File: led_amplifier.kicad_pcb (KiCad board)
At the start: 2 copper layers, 59 x 58.1 mm, 10 parts, among them J1 Conn_01x08_Female, J2 Conn_01x08_Female, Q1 IRF3205, Q2 IRF3205, Q3 IRF3205, Q4 IRF3205

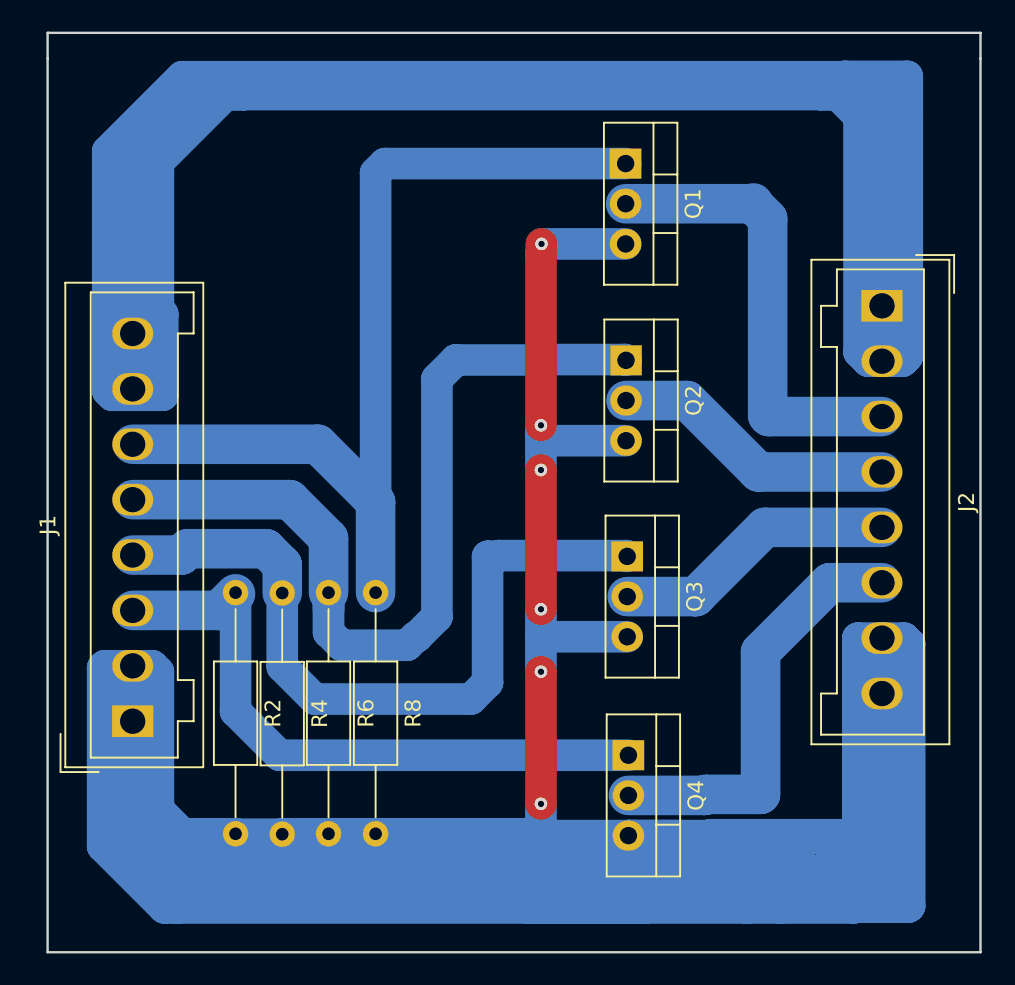
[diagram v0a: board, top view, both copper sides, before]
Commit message: Update...
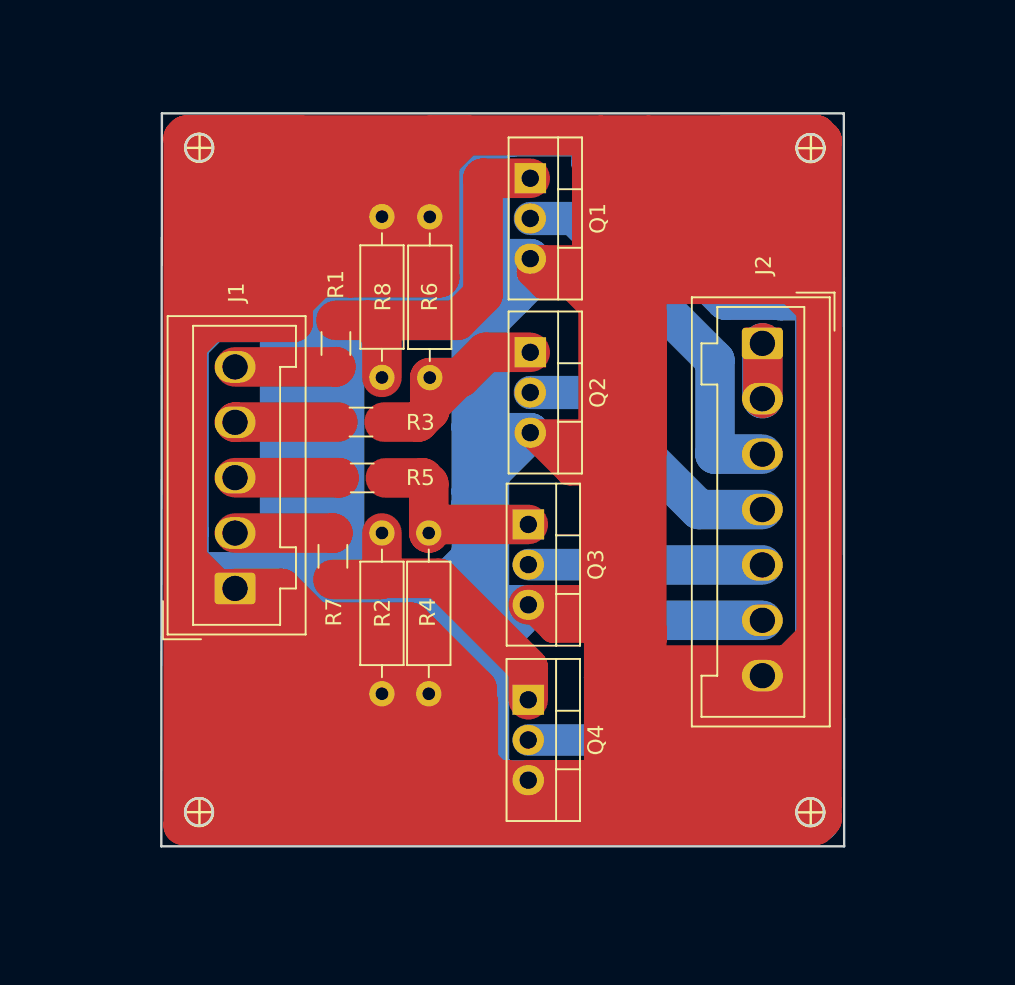
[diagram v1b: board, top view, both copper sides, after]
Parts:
- added R1: R, Resistor_SMD:R_1206_3216Metric, F.Cu at (151.9, 69.4)
- added R3: R, Resistor_SMD:R_1206_3216Metric, F.Cu at (153.5, 74.3)
- added R5: R, Resistor_SMD:R_1206_3216Metric, F.Cu at (153.6, 77.9)
- added R7: R, Resistor_SMD:R_1206_3216Metric, F.Cu at (151.8, 82.8)
- J1: value Conn_01x08_Female -> Conn_01x05; footprint Connector_Wago:Wago_734-138_1x08_P3.50mm_Vertical -> Connector_Wago:Wago_734-135_1x05_P3.50mm_Vertical
- J2: value Conn_01x08_Female -> Conn_01x07_Female; footprint Connector_Wago:Wago_734-138_1x08_P3.50mm_Vertical -> Connector_Wago:Wago_734-137_1x07_P3.50mm_Vertical
- R2, R4, R6, R8: footprint Resistor_THT:R_Axial_DIN0207_L6.3mm_D2.5mm_P15.24mm_Horizontal -> Resistor_THT:R_Axial_DIN0207_L6.3mm_D2.5mm_P10.16mm_Horizontal
- moved R6 15.0 mm to (157.9, 71.5), turned to 90 degrees
- moved R8 13.6 mm to (154.9, 71.5), turned to 90 degrees
- moved J1 10.6 mm to (145.6, 84.9)
- moved R4 10.0 mm to (157.8, 81.4)
- moved R2 9.99 mm to (154.9, 81.4)
- moved J2 7.92 mm to (178.9, 69.4)
- moved Q4 7.23 mm to (164.1, 91.9)
- moved Q3 6.57 mm to (164.1, 80.8)
- moved Q1 6.10 mm to (164.2, 58.9)
- moved Q2 6.07 mm to (164.2, 69.9)
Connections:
- J1 pad 2: Net-(J1-Pad1) -> Net-(J1-Pad2)
- J2 pad 1: Net-(J1-Pad7) -> Net-(J2-Pad1)
- J2 pad 2: Net-(J1-Pad7) -> Net-(J2-Pad1)
- Q1 pad 1: Net-(J1-Pad6) -> Net-(Q1-Pad1)
- Q2 pad 1: Net-(J1-Pad5) -> Net-(Q2-Pad1)
- Q3 pad 1: Net-(J1-Pad4) -> Net-(Q3-Pad1)
- Q4 pad 1: Net-(J1-Pad3) -> Net-(Q4-Pad1)
- R2 pad 1: Net-(J1-Pad3) -> Net-(Q4-Pad1)
- R4 pad 1: Net-(J1-Pad4) -> Net-(Q3-Pad1)
- R6 pad 1: Net-(J1-Pad5) -> Net-(Q2-Pad1)
- R8 pad 1: Net-(J1-Pad6) -> Net-(Q1-Pad1)
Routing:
- net Net-(J1-Pad1): track 434.8 -> 2789.7 mm, vias 6 -> 0
- net Net-(J1-Pad7): track 231.8 -> 0.00 mm
- net Net-(J1-Pad6): track 65.2 -> 0.00 mm
- net Net-(J1-Pad5): track 56.0 -> 6.38 mm
- net Net-(J1-Pad4): track 47.5 -> 6.50 mm
- net Net-(J1-Pad3): track 47.4 -> 6.58 mm
- net Net-(Q1-Pad1): track 0.00 -> 24.3 mm
- net Net-(J2-Pad3): track 50.8 -> 27.7 mm
- net Net-(Q4-Pad1): track 0.00 -> 19.6 mm
- net Net-(Q2-Pad1): track 0.00 -> 18.4 mm
- net Net-(Q3-Pad1): track 0.00 -> 12.5 mm
- net Net-(J2-Pad6): track 32.2 -> 20.9 mm
- net Net-(J2-Pad1): track 0.00 -> 10.5 mm
- net Net-(J2-Pad5): track 24.1 -> 14.8 mm
- net Net-(J2-Pad4): track 18.0 -> 26.0 mm
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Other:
- board size 59 x 58.1 mm -> 43.2 x 46.3 mm
- net class Default: trace_width 2.5 -> 2.1
- rule pad_to_mask_clearance: 0.2 -> 0
